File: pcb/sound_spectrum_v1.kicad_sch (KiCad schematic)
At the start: 31 parts, among them J1 SWD_CONN, J2 Conn_02x10_Counter_Clockwise, P1 USB_C_Plug_USB2.0, SW2 SW_DPST_x2, U1 STM32G473CBTx, U2 AP2112K-3.3, U3 USBLC6-2SC6

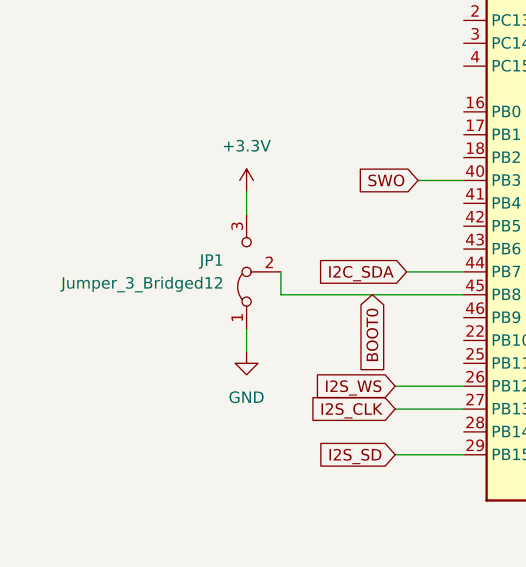
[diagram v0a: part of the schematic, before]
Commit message: chore: further tracing
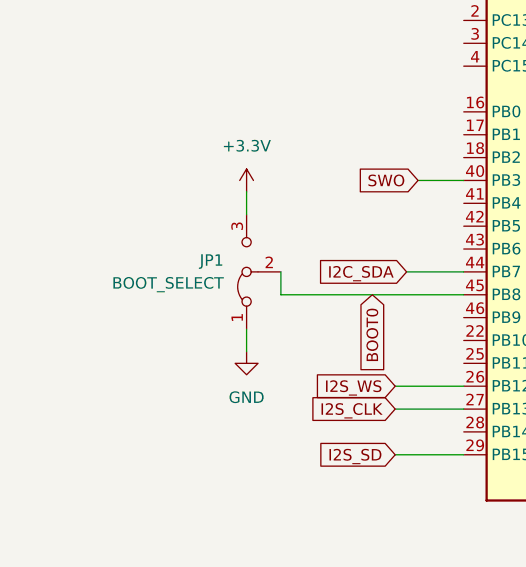
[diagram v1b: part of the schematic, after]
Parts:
- JP1: value Jumper_3_Bridged12 -> BOOT_SELECT
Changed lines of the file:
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@@
 		(on_board yes)
 		(dnp no)
-		(fields_autoplaced yes)
 		(property "Reference" "C12"
 			(at 26.67 167.6399 0)
@@
 			)
 		)
-		(property "Value" "Jumper_3_Bridged12"
+		(property "Value" "BOOT_SELECT"
 			(at 29.21 93.9799 90)
 			(effects
